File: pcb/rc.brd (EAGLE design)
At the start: 65.4 x 64.1 mm, 68 parts, among them IC2 TP4056

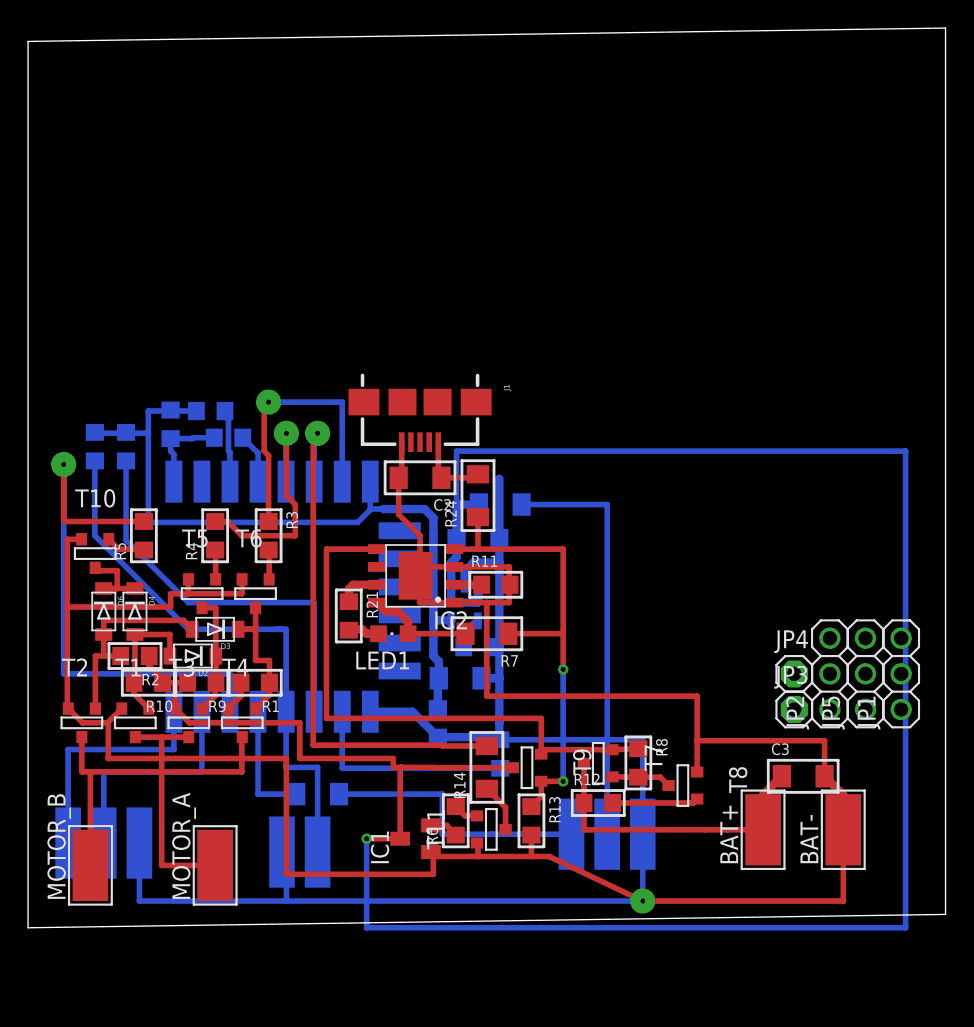
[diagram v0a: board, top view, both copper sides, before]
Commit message: pcb
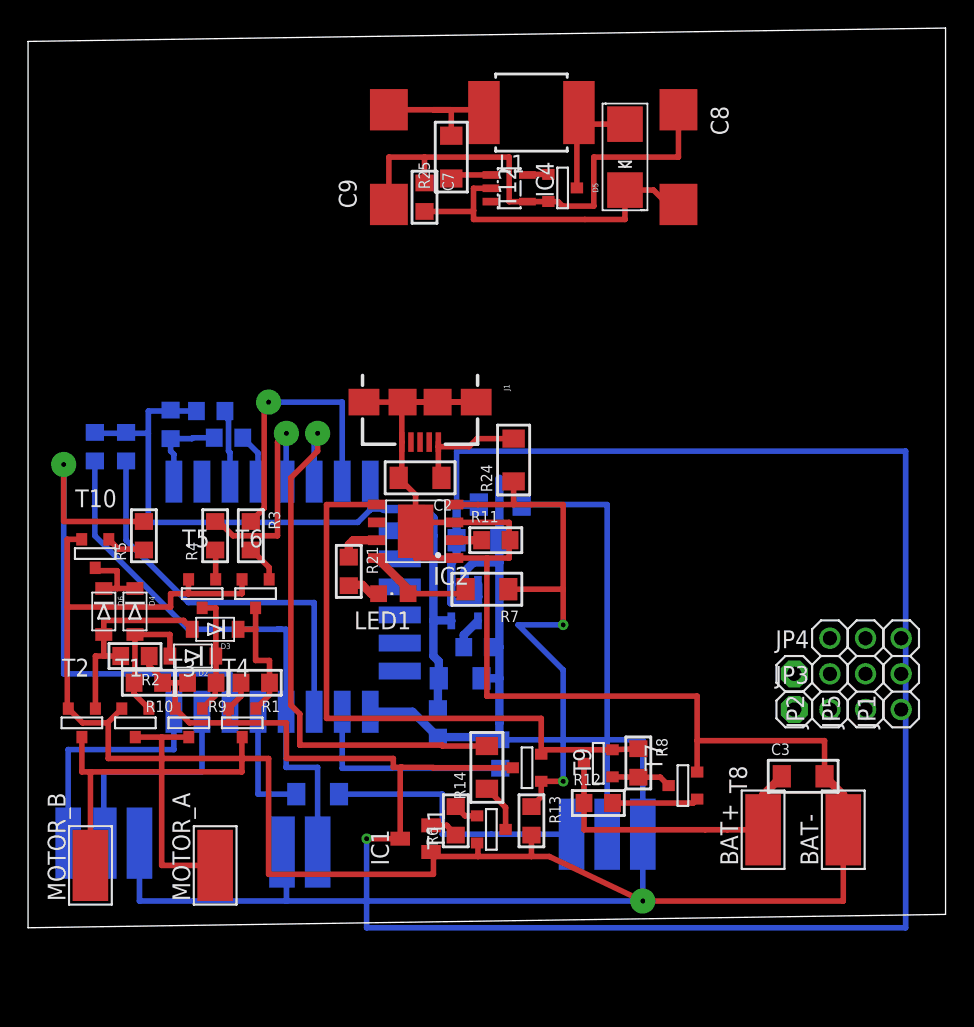
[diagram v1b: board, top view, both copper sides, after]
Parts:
- added C7: (no value), skydrop:C0805
- added C8, C9: (no value), adafruit:D/7343-31W
- added D5: (no value), adafruit:SMADIODE
- added IC4: (no value), my:SOT23-5
- added L1: (no value), inductor-neosid:MS85
- added R25: 0, skydrop:R1206
- added T12: (no value), zetex:SOT-23
- IC2: device TP4056:SOP-8 -> my:SOP-8
- moved R24 3.59 mm to (32.1, 33.0)
- moved IC2 3.18 mm to (25.1, 27.9)
- moved R11 3.18 mm to (30.8, 27.3)
- moved R21 3.18 mm to (20.3, 25.1)
- moved R7 3.18 mm to (30.2, 23.8)
- moved LED1 2.86 mm to (23.5, 23.5)
- moved R3 1.27 mm to (13.3, 27.6)
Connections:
- new net N$15: IC4.5, T12.3
- new net N$18: IC4.1, R25.1
- new net N$24: C9.+, L1.1, R25.2
- new net N$3: D5.A, L1.2, T12.1
- new net N$34: C7.2, C8.+, D5.C, IC4.2
- net GND: now also C7.1, C8.-, C9.-, IC2.HEATSINK, IC4.4, T12.2
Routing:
- net GND: track 286.0 -> 340.1 mm
- net N$34: track 0.00 -> 24.1 mm
- net N$24: track 0.00 -> 10.0 mm
- net N$3: track 0.00 -> 9.28 mm
- net V_CHRG: track 34.2 -> 41.3 mm
- net BAT_CHRG: track 40.6 -> 43.8 mm
- net N$18: track 0.00 -> 2.93 mm
- net N$10: track 5.67 -> 8.56 mm
- net BAT_CHECK: track 38.4 -> 40.3 mm
- net N$15: track 0.00 -> 1.53 mm
- net H_FWD: track 18.2 -> 16.9 mm
- net N$7: track 2.13 -> 2.67 mm

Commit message: pcb
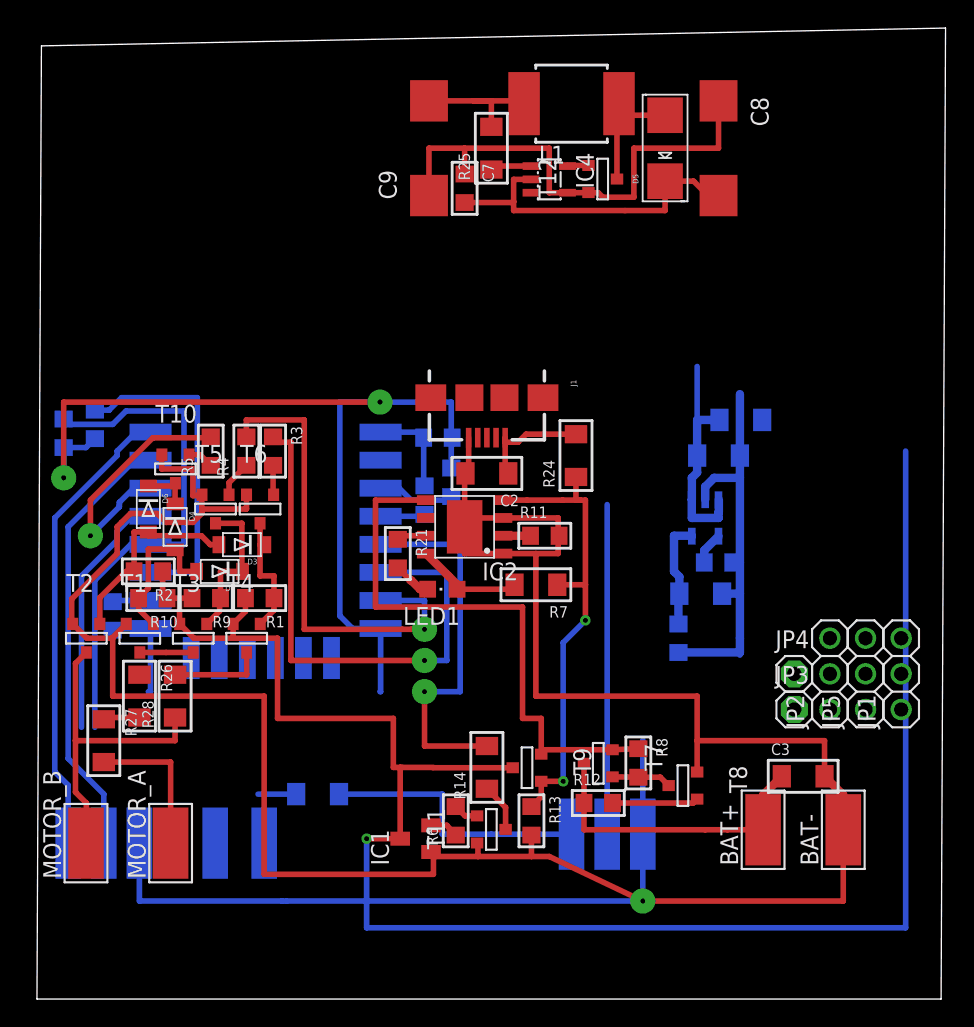
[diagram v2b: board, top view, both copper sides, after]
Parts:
- added R26, R27, R28: 0, skydrop:R1206
- moved R19 29.3 mm to (3.49, 21.9), turned to 90 degrees
- moved R15 19.1 mm to (26.7, 34.6), turned to 180 degrees
- moved C5 18.2 mm to (45.4, 23.5)
- moved C4 18.2 mm to (46.7, 25.7)
- moved C6 18.2 mm to (46.7, 33.3)
- moved IC3 18.2 mm to (45.7, 28.9)
- moved R23 18.2 mm to (48.3, 35.9)
- moved C1 18.2 mm to (43.8, 20.3)
- moved R16 17.9 mm to (27.6, 31.4), turned to 90 degrees
- moved R20 14.7 mm to (25.7, 30.2), turned to 90 degrees
- moved T10 8.31 mm to (7.94, 32.4)
- moved D6 7.96 mm to (6.03, 29.5)
- moved R5 7.69 mm to (10.5, 33.7)
- moved D4 6.68 mm to (7.94, 28.3)
- moved R4 6.43 mm to (13.0, 33.7)
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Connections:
- new net N$35: R26.2, R27.1
- new net N$36: MOTOR_A.1, R27.2
- new net N$37: R28.2, T4.1
- net BAT_CHECK: now also U1.GPIO14; no longer U1.GPIO12
- net H_BCK: now also U1.GPIO12; no longer U1.GPIO13
- net H_FWD: now also U1.GPIO13; no longer U1.GPIO14
- net N$33: now also R26.1; no longer MOTOR_A.1
- net N$4: now also R28.1; no longer T4.1
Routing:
- net GND: track 340.1 -> 308.8 mm
- net BAT_PROT: track 171.4 -> 144.6 mm
- net VCC: track 53.7 -> 76.6 mm, vias 0 -> 2
- net H_PWM: track 39.3 -> 18.9 mm
- net H_BCK: track 20.0 -> 39.6 mm
- net H_FWD: track 16.9 -> 34.3 mm
- net TX: track 16.9 -> 33.1 mm
- net RX: track 16.7 -> 31.8 mm
- net BAT_CHECK: track 40.3 -> 27.0 mm
- net N$33: track 16.8 -> 3.81 mm
- net N$26: track 15.3 -> 3.23 mm
- net SERVO_CONTROL: track 8.59 -> 20.6 mm
- net N$36: track 0.00 -> 10.5 mm
- net V_CHRG: track 41.3 -> 33.9 mm
- net N$37: track 0.00 -> 6.69 mm
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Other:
- board size 65.4 x 64.1 mm -> 64.8 x 69.2 mm

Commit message: pcb
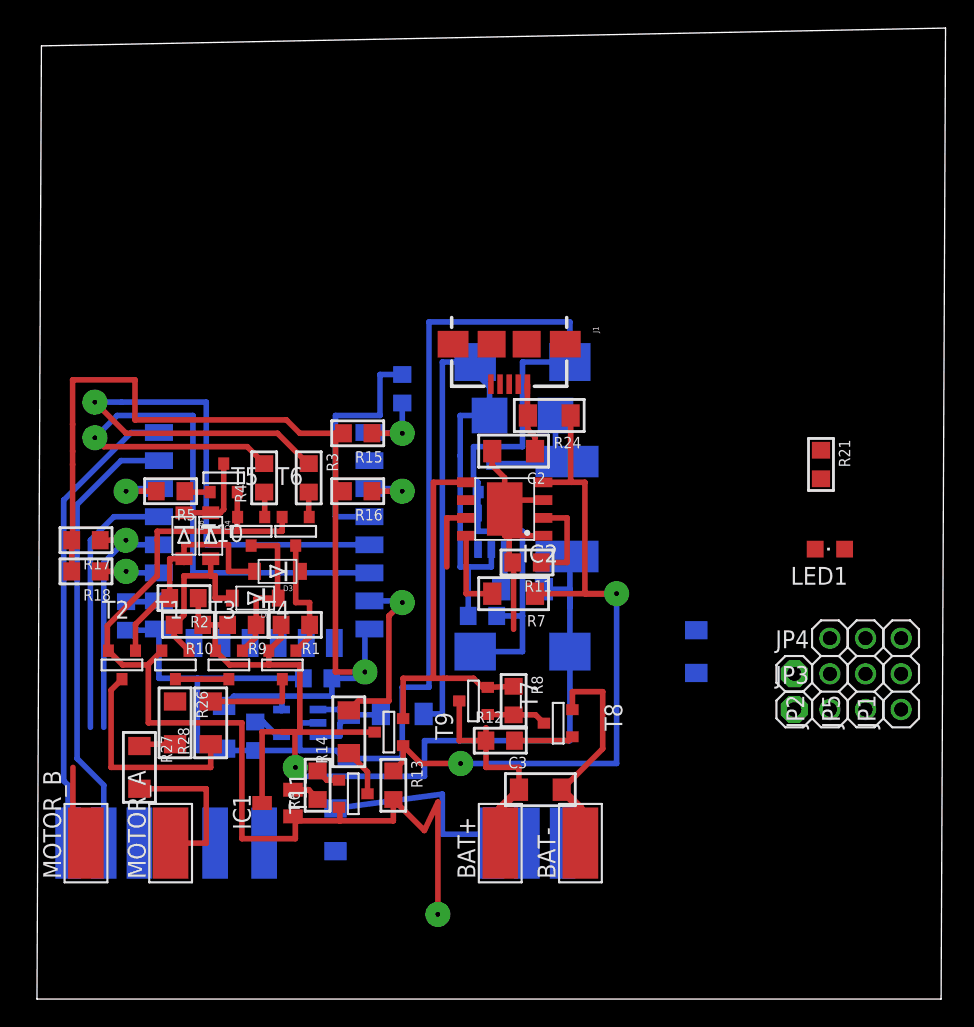
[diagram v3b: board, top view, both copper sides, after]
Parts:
- added R29: 0, skydrop:R1206
- U1: device esp8266modules:ESP12E-SMD -> my:ESP-12
- moved C9 36.5 mm to (32.7, 19.4), flipped to the bottom, turned to 180 degrees
- moved C5 35.3 mm to (11.4, 14.0), turned to 270 degrees
- moved C4 35.3 mm to (13.7, 13.3), turned to 90 degrees
- moved C6 33.1 mm to (20.3, 13.3), turned to 270 degrees
- moved IC3 32.4 mm to (16.8, 14.3), turned to 270 degrees
- moved R25 31.5 mm to (32.7, 23.8), flipped to the bottom, turned to 180 degrees
- moved R21 30.8 mm to (54.0, 32.7)
- moved C7 30.5 mm to (29.8, 21.9), flipped to the bottom, turned to 0 degrees
- moved L1 28.9 mm to (35.9, 29.5), flipped to the bottom, turned to 0 degrees
- moved LED1 27.8 mm to (54.6, 26.7)
- moved C1 25.9 mm to (18.1, 17.5), turned to 180 degrees
- moved IC4 25.4 mm to (30.5, 27.9), flipped to the bottom, turned to 0 degrees
- moved T12 22.7 mm to (30.5, 31.8), flipped to the bottom, turned to 180 degrees
- moved D5 21.6 mm to (32.7, 36.2), flipped to the bottom, turned to 180 degrees
- moved C8 20.7 mm to (32.7, 40.0), flipped to the bottom, turned to 0 degrees
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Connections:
- removed net N$34: C7.2, C8.+, D5.C, IC4.2
- new net 5V: C7.2, C8.+, D5.C, IC4.2, R23.2, R29.2
- net BAT_CHECK: now also U1.GPIO13; no longer U1.GPIO14
- net BAT_PROT: now also C9.+, L1.1, R25.2; no longer C6.1, IC3.1, IC3.3, R23.2
- net H_BCK: now also U1.GPIO14; no longer U1.GPIO12
- net H_FWD: now also U1.GPIO12; no longer U1.GPIO13
- net N$24: now also C6.1, IC3.1, IC3.3, R29.1; no longer C9.+, L1.1, R25.2
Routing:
- net BAT_PROT: track 144.6 -> 76.5 mm
- net GND: track 308.8 -> 242.2 mm
- net 5V: track 0.00 -> 52.9 mm
- net N$34: track 24.1 -> 0.00 mm
- net N$30: track 23.5 -> 0.00 mm
- net V_CHRG: track 33.9 -> 53.8 mm
- net N$22: track 23.9 -> 4.29 mm, vias 0 -> 1
- net N$21: track 37.3 -> 19.3 mm, vias 0 -> 1
- net H_PWM: track 18.9 -> 4.58 mm
- net BAT_CHECK: track 27.0 -> 13.0 mm
- net N$23: track 3.40 -> 17.3 mm
- net BAT_CHRG: track 40.6 -> 27.3 mm
- net H_FWD: track 34.3 -> 44.8 mm
- net H_BCK: track 39.6 -> 47.4 mm
- net BAT+: track 23.8 -> 17.8 mm
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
